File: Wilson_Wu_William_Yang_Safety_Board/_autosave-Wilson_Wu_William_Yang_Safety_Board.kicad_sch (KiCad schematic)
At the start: 59 parts, among them J1 22035035, J2 XT60-M, J3 XT60-M, J4 M22-7130442, J6 430450200, J7 430450200, J8 430450200, Q1 IRLML6344TRPBF, U1 STM32, U10 10kohm, U11 LMV331IDBVR, U13 SN74AHCT14QPWRQ1, U2 MCP2562-E_P, U3 MCP6286T-E/OT, U4 SN74HCS21QPWRQ1, U6 J115F11AH12VDCS61.5U

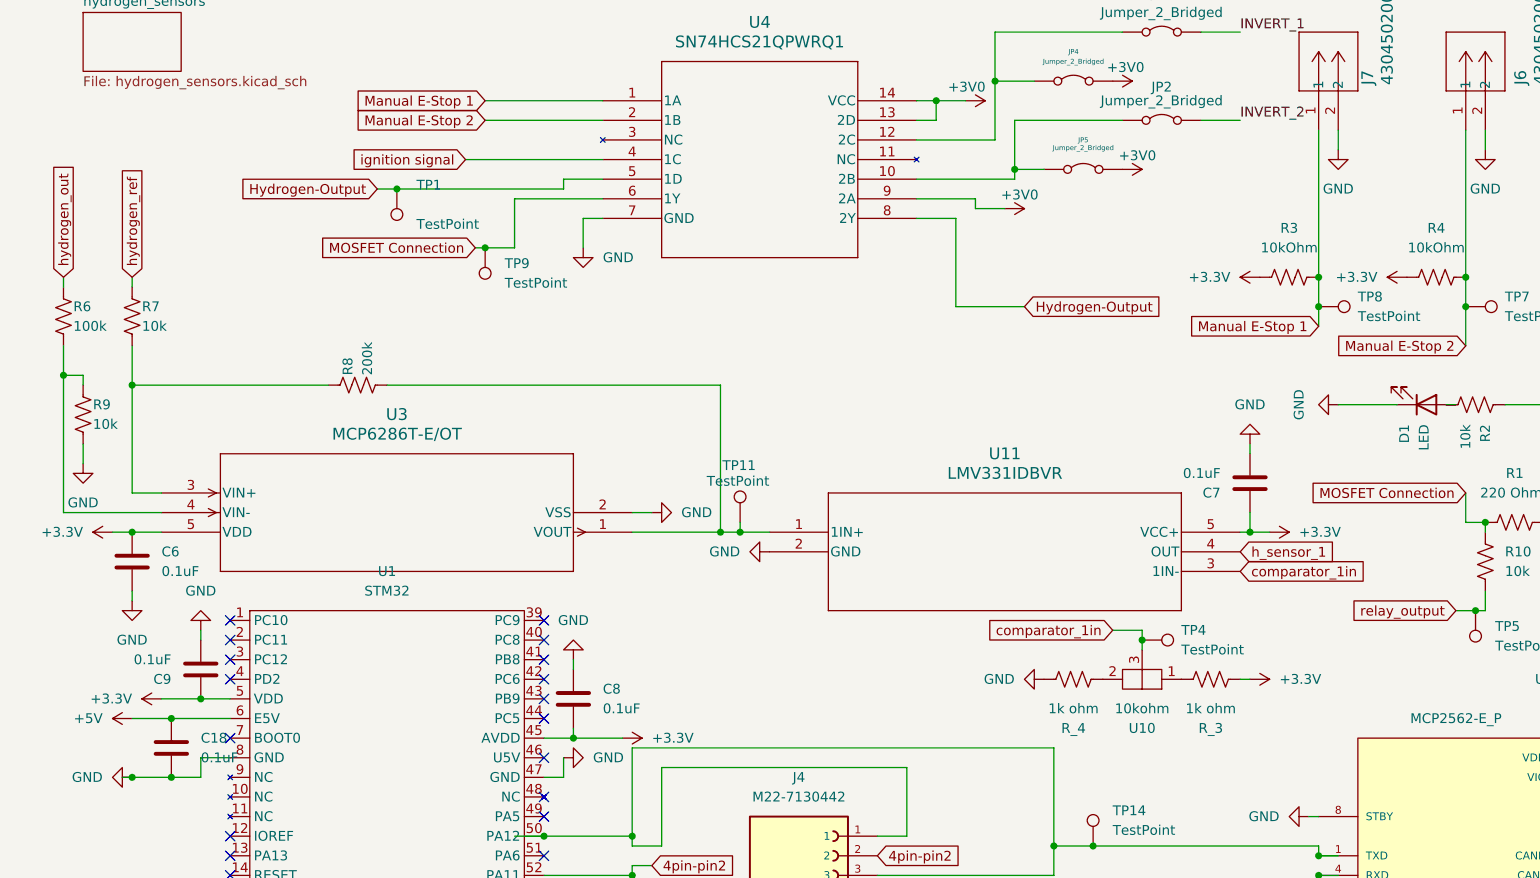
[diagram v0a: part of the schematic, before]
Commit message: sch changes
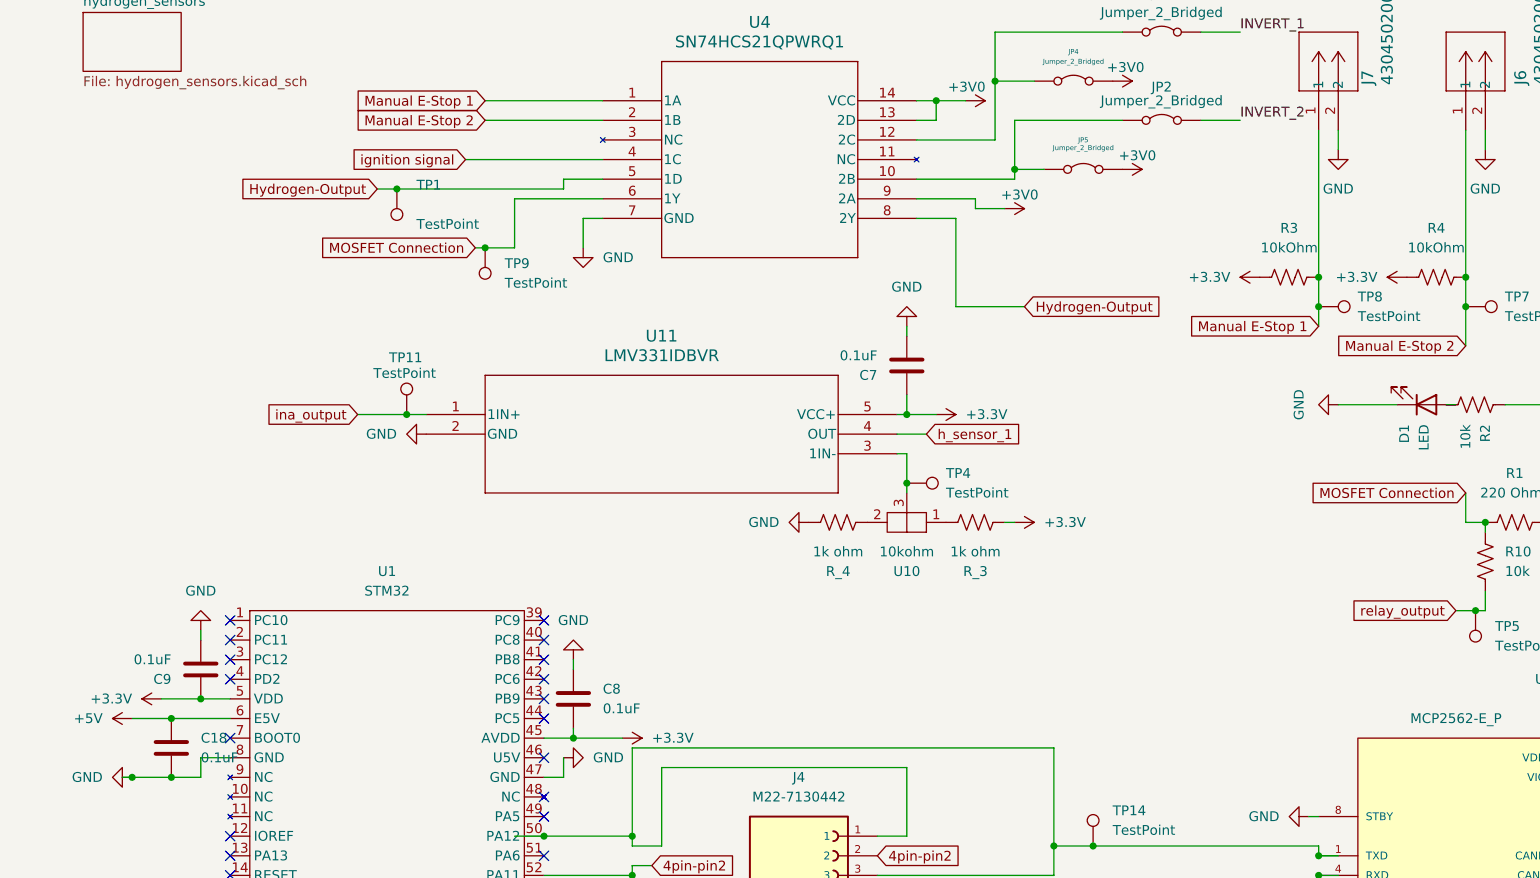
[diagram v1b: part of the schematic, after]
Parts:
- removed C6: 0.1uF, Capacitor_SMD:C_0805_2012Metric, symbol Device:C
- removed R6: 100k, Resistor_SMD:R_0805_2012Metric, symbol Device:R_US
- removed R7, R9: 10k, Resistor_SMD:R_0805_2012Metric, symbol Device:R_US
- removed R8: 200k, Resistor_SMD:R_0805_2012Metric, symbol Device:R_US
- removed U3: MCP6286T-E/OT, SMV_ICs:SOT-23-5_MC_MCH, symbol SMV_Custom_Updated:MCP6286T-E_OT
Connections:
- net ina_output: now reaches TP11.1, U11.1 (1IN+)
- net comparator_1in: no longer names the net of TP4.1, U10.3, U11.3 (1IN-)
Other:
- moved on the sheet: C7, R_3, R_4, TP11, TP4, U10, U11
